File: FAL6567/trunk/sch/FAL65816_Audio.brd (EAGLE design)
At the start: 31 parts, among them IC1 74LS688DW, IC2 74LS00D, Q1 2N2222, U2 65C22

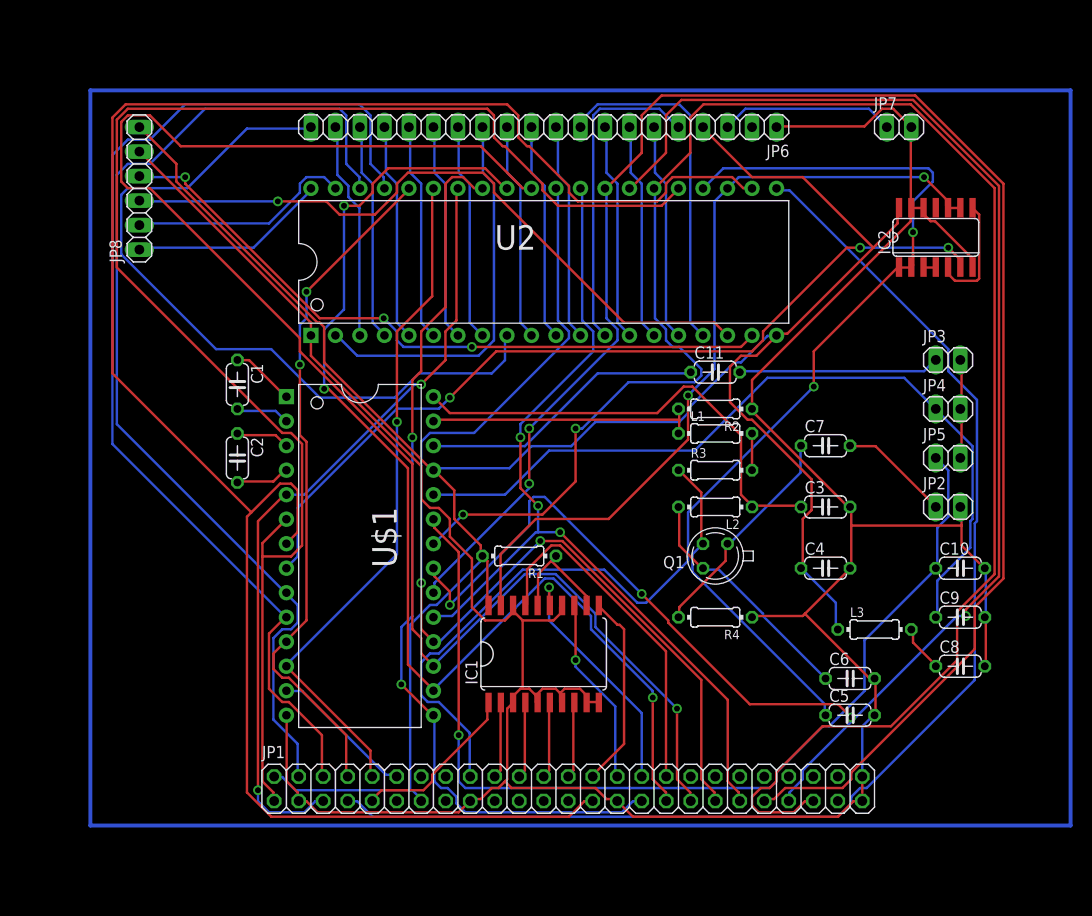
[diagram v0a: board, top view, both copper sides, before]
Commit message: FAL65816 - update
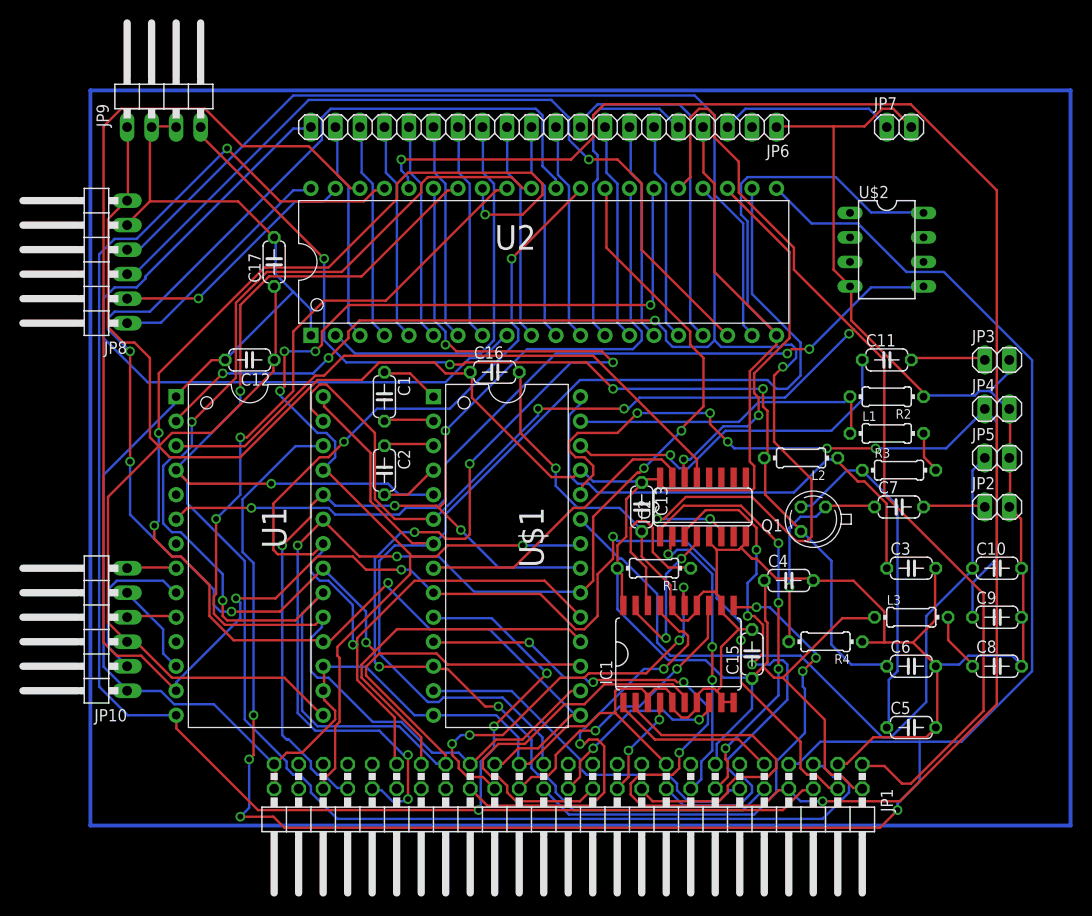
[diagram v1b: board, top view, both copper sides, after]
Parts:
- added C12, C13, C15, C16: 0.1, resistor:C050-024X044
- added C17: 10, resistor:C050-024X044
- added JP10: 5V Serial Port, pinhead:1X06/90
- added JP9: POWER, pinhead:1X04/90
- added U$2: OSC, FT74xx:DIL08
- added U1: 65C51, 65xxx:DIP-28
- IC2: value 74LS00D -> 74LS138D; device FT74xx:SO14 -> FT74xx:SO16
- JP1: device pinhead:2X25 -> pinhead:2X25/90
- JP2: value (none) -> AUDIO OUT
- JP3: value (none) -> EXT IN
- JP4: value (none) -> POTX
- JP5: value (none) -> POTY
- JP6: value (none) -> KEYBOARD PORT
- JP8: device pinhead:1X06 -> pinhead:1X06/90
- moved IC2 36.9 mm to (63.5, 33.0)
- moved R3 19.0 mm to (83.8, 36.8)
- moved C11 17.8 mm to (82.5, 48.3)
- moved R2 17.8 mm to (82.5, 44.5)
- moved L1 17.8 mm to (82.5, 40.6)
- moved C1 15.3 mm to (30.5, 44.5)
- moved C2 15.3 mm to (30.5, 36.8)
- moved U$1 15.2 mm to (43.2, 29.2)
- moved R1 14.0 mm to (58.4, 26.7)
- moved IC1 14.0 mm to (61.0, 17.8)
- moved R4 11.7 mm to (76.2, 19.1)
- moved C3 10.9 mm to (85.1, 26.7)
- moved Q1 10.9 mm to (74.9, 31.8)
- moved L2 10.2 mm to (73.7, 38.1)
- moved C7 9.92 mm to (83.8, 33.0)
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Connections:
- removed net N$10: JP3.2, JP4.2, JP5.2
- removed net N$14: IC2.5, IC2.8
- removed net N$15: IC1.12, IC1.16, R1.1
- new net CS6522N: IC2.14, U2.23
- new net CS6551N: IC2.13, U1.3
- new net N$20: JP10.4, U1.10
- new net N$21: JP10.5, U1.12
- new net N$22: JP10.6, U1.8
- new net N$28: U$2.5, U1.6
- new net PU1: IC1.18, IC2.6, R1.1, U1.2, U2.24
- net +12V: now also JP9.4
- net A0: now also U1.13
- net A1: now also U1.14
- net A5: now also IC2.1
- net A6: now also IC2.2
- net A7: now also IC2.3; no longer IC2.1, IC2.2, U2.24
- net CS6581N: now also IC2.15; no longer IC2.6
- net CSN: now also IC2.4; no longer IC2.10, IC2.9, U2.23
- net D0: now also U1.18
- net D1: now also U1.19
- net D2: now also U1.20
- net D3: now also U1.21
- net D4: now also U1.22
- net D5: now also U1.23
- net D6: now also U1.24
- net D7: now also U1.25
- net GND: now also C12.2, C13.2, C15.2, C16.2, C17.2, IC1.12, IC1.16, IC2.5, IC2.8, JP10.1, JP3.2, JP4.2, JP5.2, JP9.2, JP9.3, U$2.4, U1.1, U1.16, U1.17; no longer IC1.18, IC2.12, IC2.13, IC2.7
- net IRQN: now also U1.26
- net N$17: now also JP10.2, U1.9; no longer IC2.3, IC2.4
- net PH2: now also U1.27
- net RESN: now also U1.4
- net RW: now also U1.28
- net VCC: now also C12.1, C13.1, C15.1, C16.1, C17.1, IC2.16, JP10.3, JP9.1, U$2.8, U1.15; no longer IC2.14
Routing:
- net PU1: track 0.00 -> 156.7 mm, vias 0 -> 6
- net A2: track 71.0 -> 215.5 mm, vias 2 -> 6
- net VCC: track 232.1 -> 350.0 mm
- net RESN: track 81.4 -> 178.3 mm
- net A0: track 107.9 -> 199.1 mm, vias 0 -> 4
- net N$28: track 0.00 -> 90.2 mm, vias 0 -> 3
- net GND: track 325.5 -> 414.6 mm, vias 0 -> 1
- net +12V: track 25.1 -> 111.7 mm, vias 0 -> 4
- net IRQN: track 132.3 -> 217.3 mm, vias 0 -> 4
- net A1: track 113.0 -> 194.1 mm, vias 0 -> 4
- net RW: track 200.8 -> 129.5 mm
- net D6: track 183.5 -> 114.8 mm
- net A7: track 125.9 -> 57.3 mm, vias 2 -> 3
- net CSN: track 83.7 -> 16.8 mm
- net CS6551N: track 0.00 -> 64.2 mm
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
